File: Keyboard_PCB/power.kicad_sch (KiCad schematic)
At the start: 13 parts, among them Q1 AO3401A

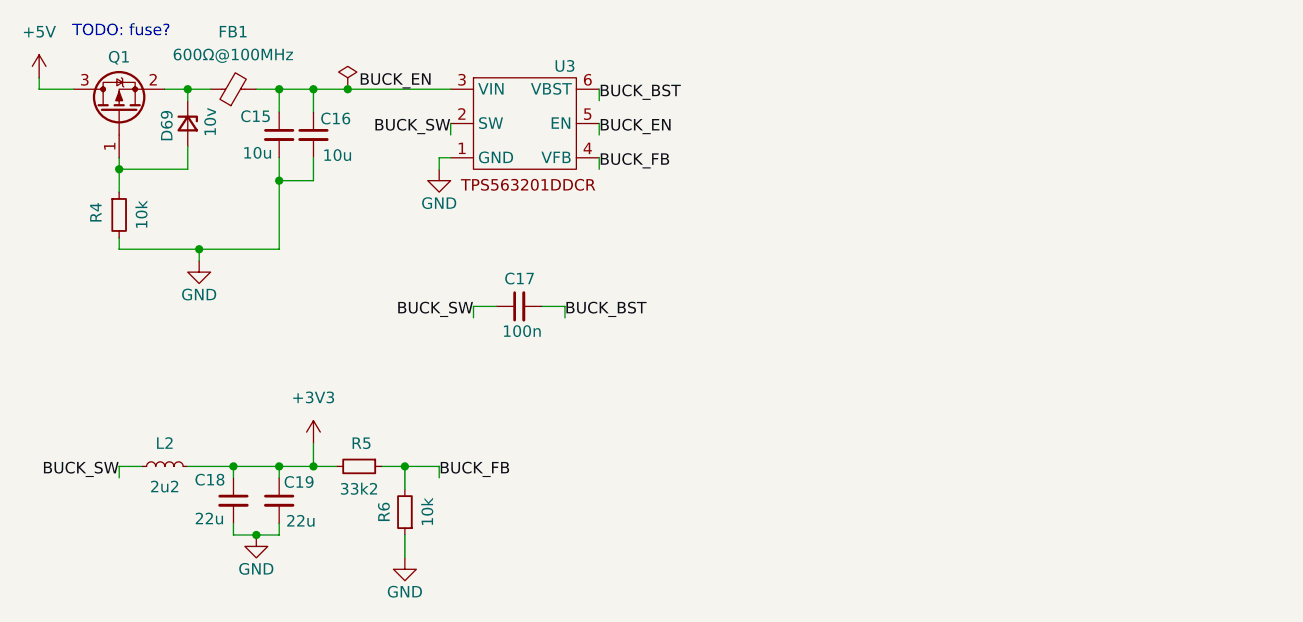
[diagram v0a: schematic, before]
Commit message: Layout Progress
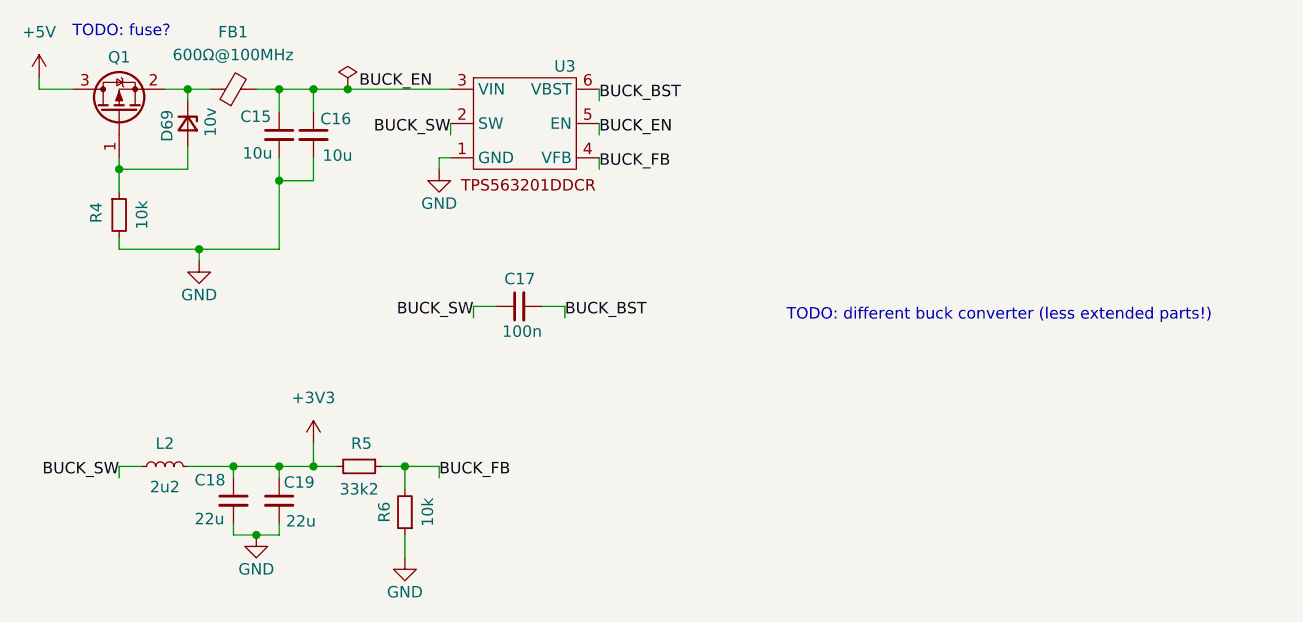
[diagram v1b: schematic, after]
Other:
- note added: "TODO: different buck converter (less extended parts!)"
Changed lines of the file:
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@@
+		)
+	)
+	(text "TODO: different buck converter (less extended parts!)"
+		(exclude_from_sim no)
+		(at 140.97 59.436 0)
+		(effects
+			(font
+				(size 1.27 1.27)
+			)
 		)
 	)

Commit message: Layout V1
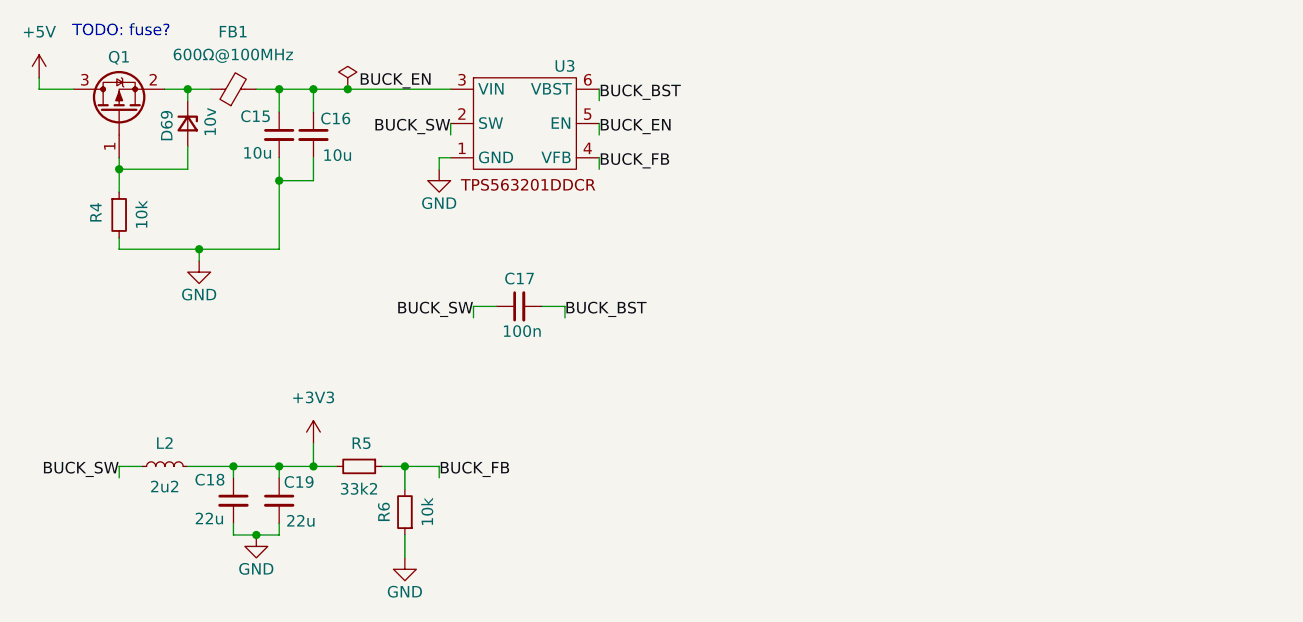
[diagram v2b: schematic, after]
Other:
- note removed: "TODO: different buck converter (less extended parts!)"
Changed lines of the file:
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@@
-		)
-	)
-	(text "TODO: different buck converter (less extended parts!)"
-		(exclude_from_sim no)
-		(at 140.97 59.436 0)
-		(effects
-			(font
-				(size 1.27 1.27)
-			)
 		)
 	)
